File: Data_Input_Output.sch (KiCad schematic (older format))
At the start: 38 parts, among them K1 G5LE_1A4_DC3, K2 G5LE_1A4_DC3, P10 CONN_01X02, P11 CONN_01X02, P12 CONN_01X02, P3 CONN_01X04, P4 CONN_01X04, P5 CONN_01X04, P6 CONN_01X04, P7 CONN_01X02, P8 CONN_01X02, P9 CONN_01X02, Q1 2N7002K, Q2 2N7002K, Q3 BSS215PH6327, Q4 Si5468DC, Q5 Si5468DC, Q6 Si5468DC, U11 MCP2551-I/SN, U12 ST1480ABDR, U13 SCHA4B0419

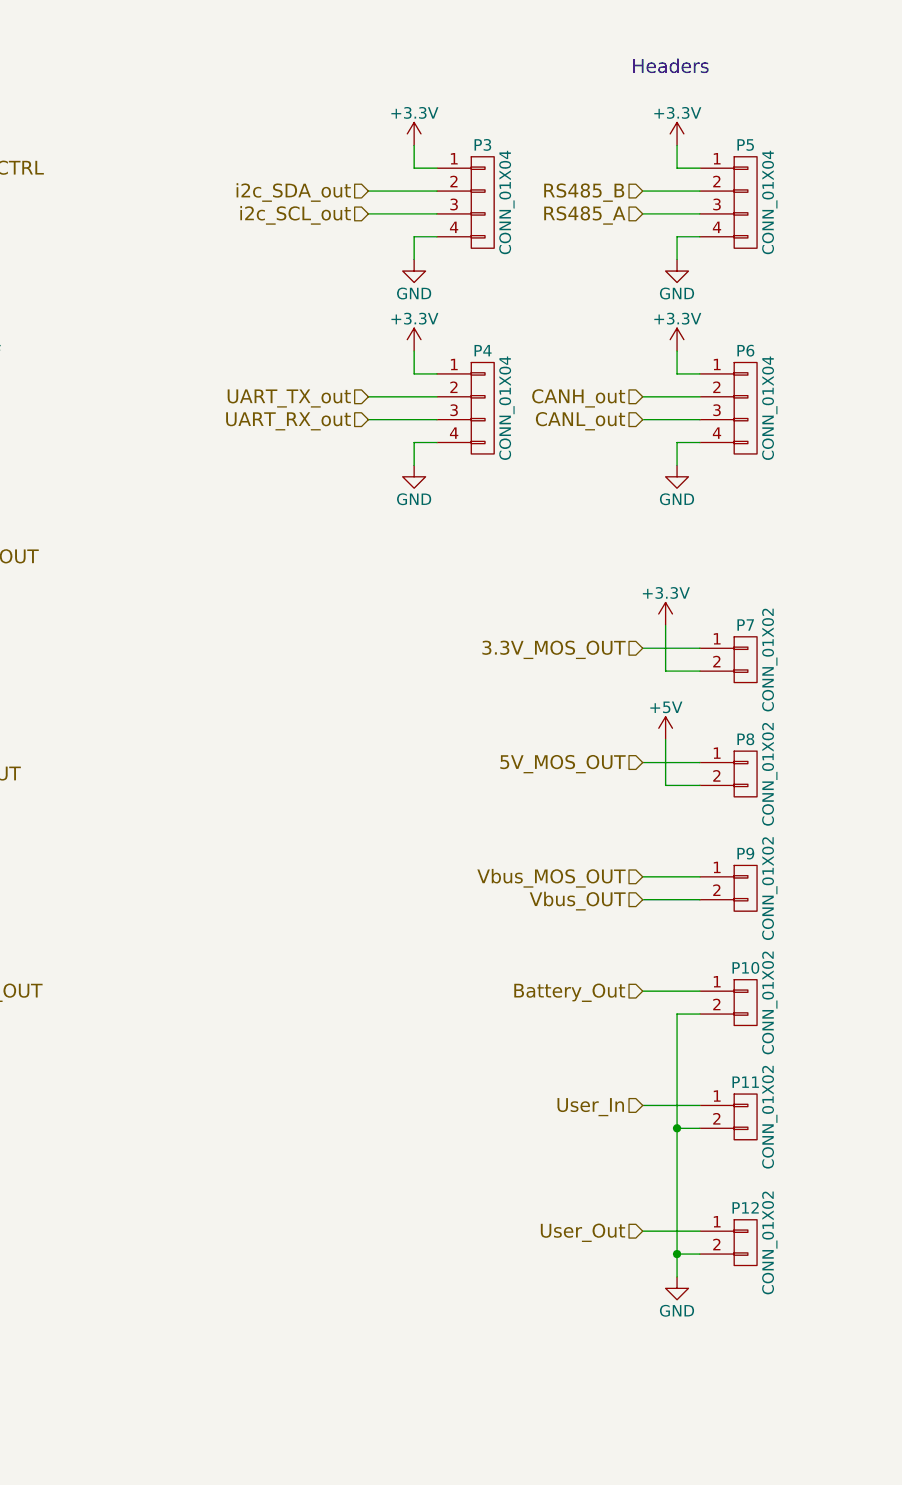
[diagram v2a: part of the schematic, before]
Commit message: board layout 95% complete
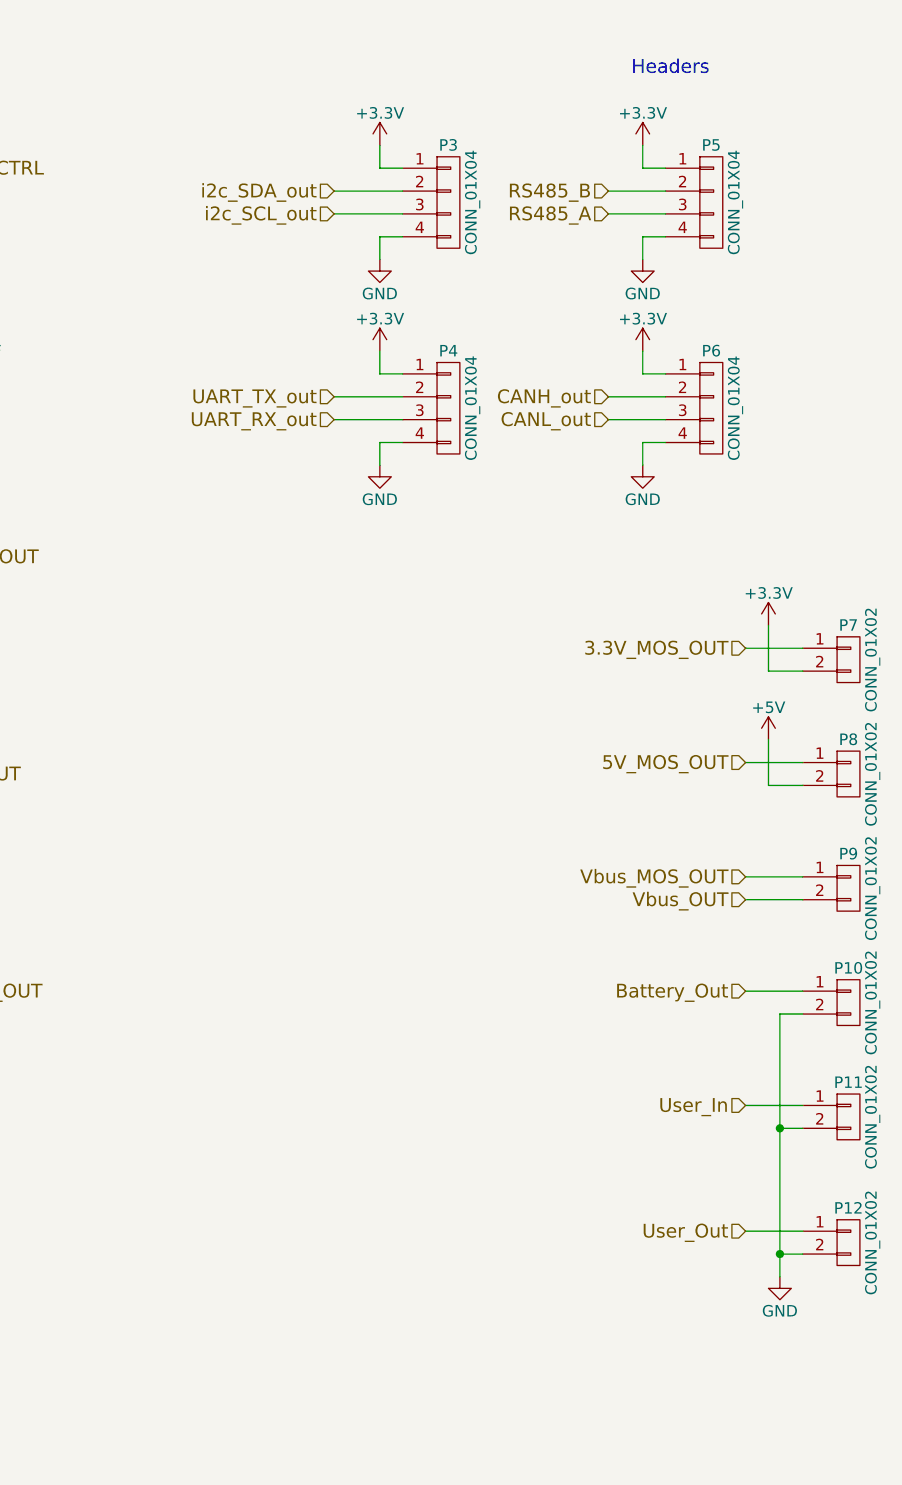
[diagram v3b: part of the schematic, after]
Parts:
- U13: footprint SPEX_Parts:SCHA4B0400 -> SPEX_Parts:SCH4B0419
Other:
- moved on the sheet: P10, P11, P12, P3, P4, P5, P6, P7, P8, P9
